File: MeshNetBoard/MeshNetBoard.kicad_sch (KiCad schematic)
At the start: 9 parts, among them J1 Conn_01x02, U1 XIAO-ESP32-S3-DIP, U2 TPS631000DRLR

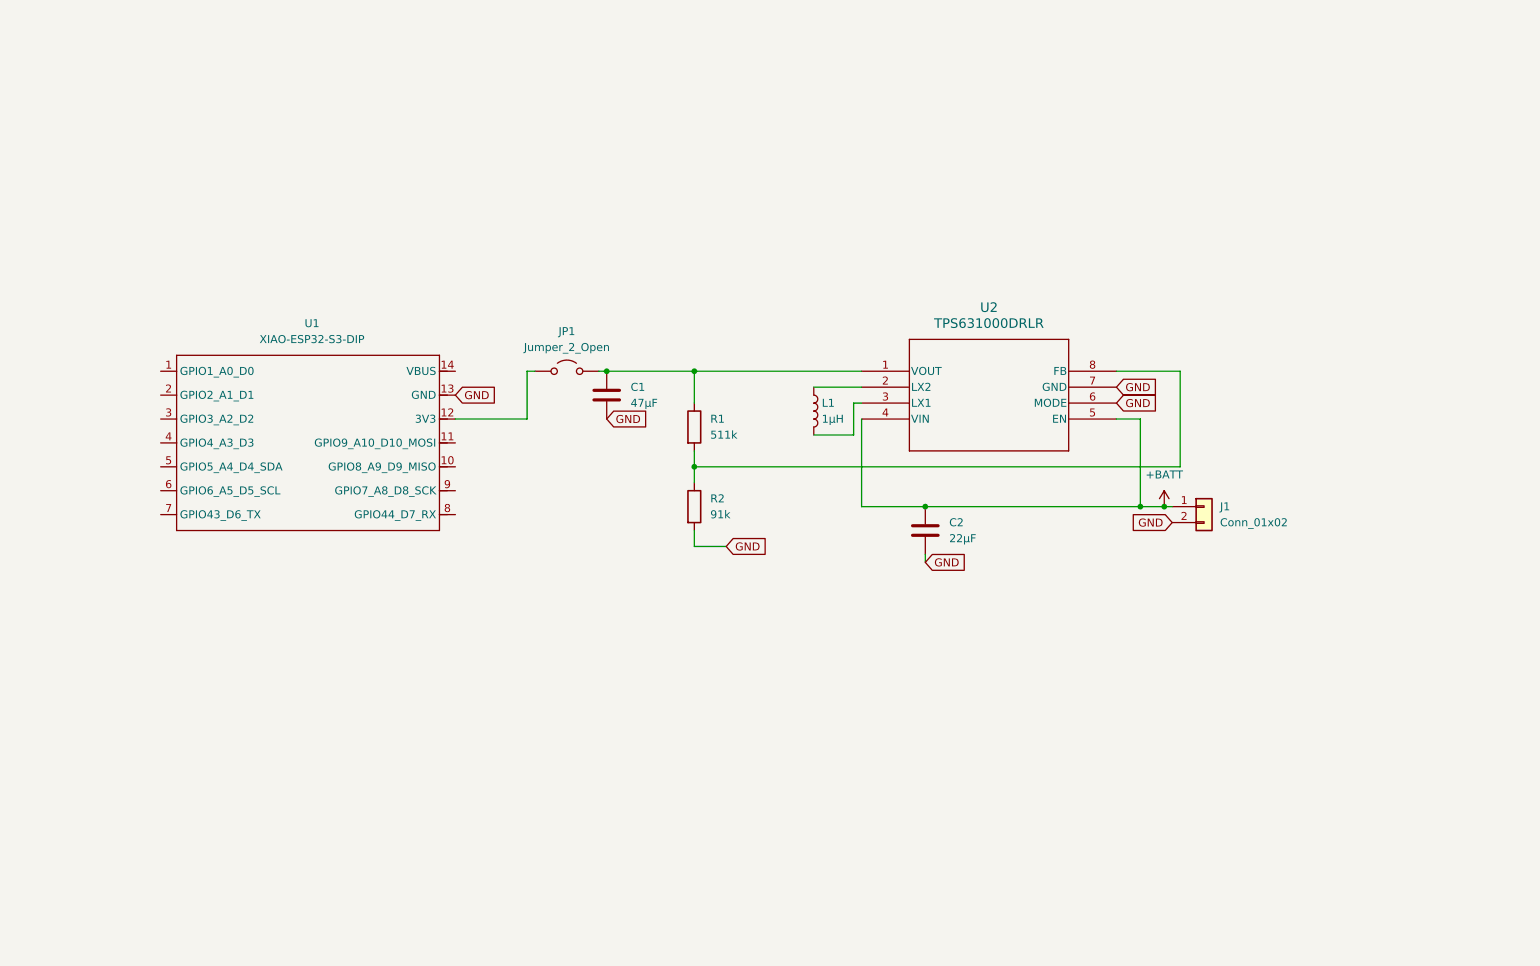
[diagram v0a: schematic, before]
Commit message: for pdr
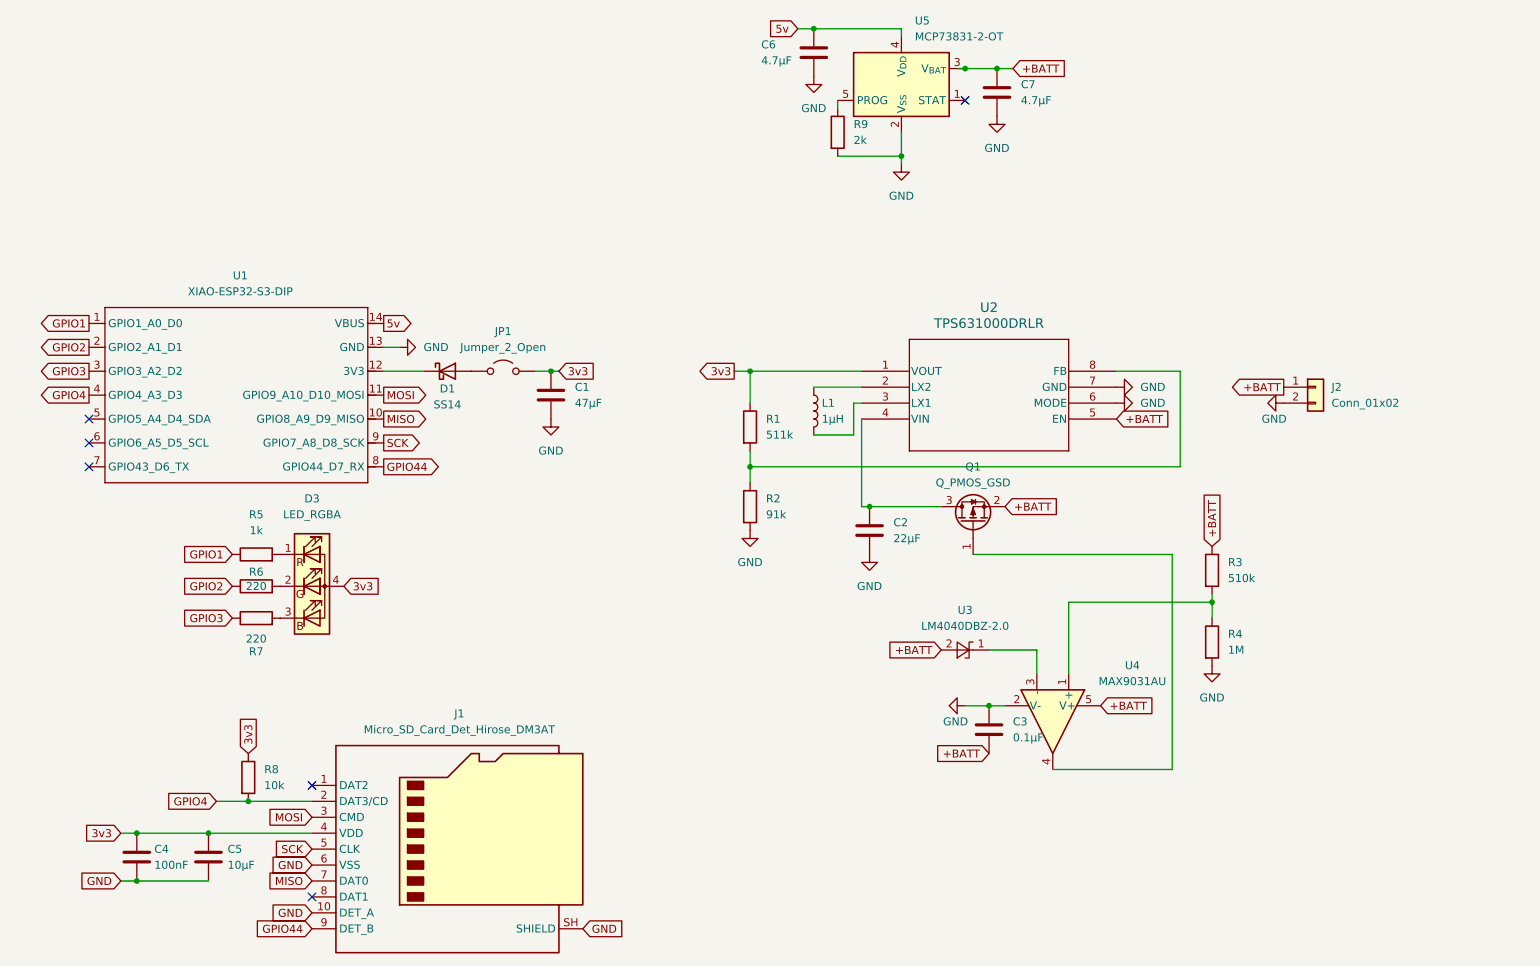
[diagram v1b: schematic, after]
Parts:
- removed J1: Conn_01x02, Connector_JST:JST_PH_S2B-PH-K_1x02_P2.00mm_Horizontal, symbol Connector_Generic:Conn_01x02
- added C3: 0.1μF, Capacitor_SMD:C_0805_2012Metric_Pad1.18x1.45mm_HandSolder, symbol Device:C
- added C4: 100nF, Capacitor_SMD:C_0805_2012Metric_Pad1.18x1.45mm_HandSolder, symbol Device:C
- added C5: 10µF, Capacitor_SMD:C_0805_2012Metric_Pad1.18x1.45mm_HandSolder, symbol Device:C
- added C6, C7: 4.7µF, Capacitor_SMD:C_0805_2012Metric_Pad1.18x1.45mm_HandSolder, symbol Device:C
- added D1: SS14, Diode_SMD:D_SMA, symbol Diode:SS14
- added D3: LED_RGBA, symbol Device:LED_RGBA
- added J1: Micro_SD_Card_Det_Hirose_DM3AT, symbol Connector:Micro_SD_Card_Det_Hirose_DM3AT
- added J2: Conn_01x02, Connector_JST:JST_PH_S2B-PH-K_1x02_P2.00mm_Horizontal, symbol Connector_Generic:Conn_01x02
- added Q1: Q_PMOS_GSD, Package_TO_SOT_SMD:SOT-23, symbol Transistor_FET:Q_PMOS_GSD
- added R3: 510k, Resistor_SMD:R_0805_2012Metric_Pad1.20x1.40mm_HandSolder, symbol Device:R
- added R4: 1M, Resistor_SMD:R_0805_2012Metric_Pad1.20x1.40mm_HandSolder, symbol Device:R
- added R5: 1k, Resistor_SMD:R_0805_2012Metric_Pad1.20x1.40mm_HandSolder, symbol Device:R
- added R6, R7: 220, Resistor_SMD:R_0805_2012Metric_Pad1.20x1.40mm_HandSolder, symbol Device:R
- added R8: 10k, Resistor_SMD:R_0805_2012Metric_Pad1.20x1.40mm_HandSolder, symbol Device:R
- added R9: 2k, Resistor_SMD:R_0805_2012Metric_Pad1.20x1.40mm_HandSolder, symbol Device:R
- added U3: LM4040DBZ-2.0, Package_TO_SOT_SMD:SOT-23, symbol Reference_Voltage:LM4040DBZ-2.0
- added U4: MAX9031AU, Package_TO_SOT_SMD:SOT-23-5, symbol Comparator:MAX9031AU
- added U5: MCP73831-2-OT, Package_TO_SOT_SMD:SOT-23-5, symbol Battery_Management:MCP73831-2-OT
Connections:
- net +BATT: now also C3.2, C7.1, J2.1 (Pin_1), Q1.2 (S), R3.1, U3.2 (A), U4.5 (V+), U5.3 (V_{BAT}); no longer C2.1, U2.4 (VIN)
- net GND: now also C3.1, C4.2, C5.2, C6.2, C7.2, J1.10 (DET_A), J1.6 (VSS), J1.SH (SHIELD), J2.2 (Pin_2), R4.2, R9.2, U4.2 (V-), U5.2 (V_{SS})
- net 3v3: now reaches C1.1, JP1.2 (B), R1.1, U2.1 (VOUT)
- net 3v3: now also C4.1, C5.1, D3.4 (A), J1.4 (VDD), R8.1
- net at U1.12 (3V3): now also D1.1 (K); no longer JP1.1 (A)
- net GPIO1: now reaches U1.1 (GPIO1_A0_D0)
- net GPIO1: now also R5.1
- net MISO: now reaches U1.10 (GPIO8_A9_D9_MISO)
- net MISO: now also J1.7 (DAT0)
- net MOSI: now reaches U1.11 (GPIO9_A10_D10_MOSI)
- net MOSI: now also J1.3 (CMD)
- net 5v: now reaches U1.14 (VBUS)
- net 5v: now also C6.1, U5.4 (V_{DD})
- net GPIO2: now reaches U1.2 (GPIO2_A1_D1)
- net GPIO2: now also R6.1
- net GPIO3: now reaches U1.3 (GPIO3_A2_D2)
- net GPIO3: now also R7.1
- net GPIO4: now reaches U1.4 (GPIO4_A3_D3)
- net GPIO4: now also J1.2 (DAT3/CD), R8.2
- net GPIO44: now reaches U1.8 (GPIO44_D7_RX)
- net GPIO44: now also J1.9 (DET_B)
- net SCK: now reaches U1.9 (GPIO7_A8_D8_SCK)
- net SCK: now also J1.5 (CLK)
- new net: D1.2 (A), JP1.1 (A)
- new net: R3.2, R4.1, U4.1 (+)
- new net: U3.1 (K), U4.3 (-)
- new net: Q1.1 (G), U4.4
- new net: D3.3 (BK), R7.2
- new net: D3.2 (GK), R6.2
- new net: C2.1, Q1.3 (D), U2.4 (VIN)
- new net: R9.1, U5.5 (PROG)
- new net: D3.1 (RK), R5.2
- no-connect marks 0 -> 6
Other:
- moved on the sheet: C1, C2, JP1, R1, R2, U1

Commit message: help me
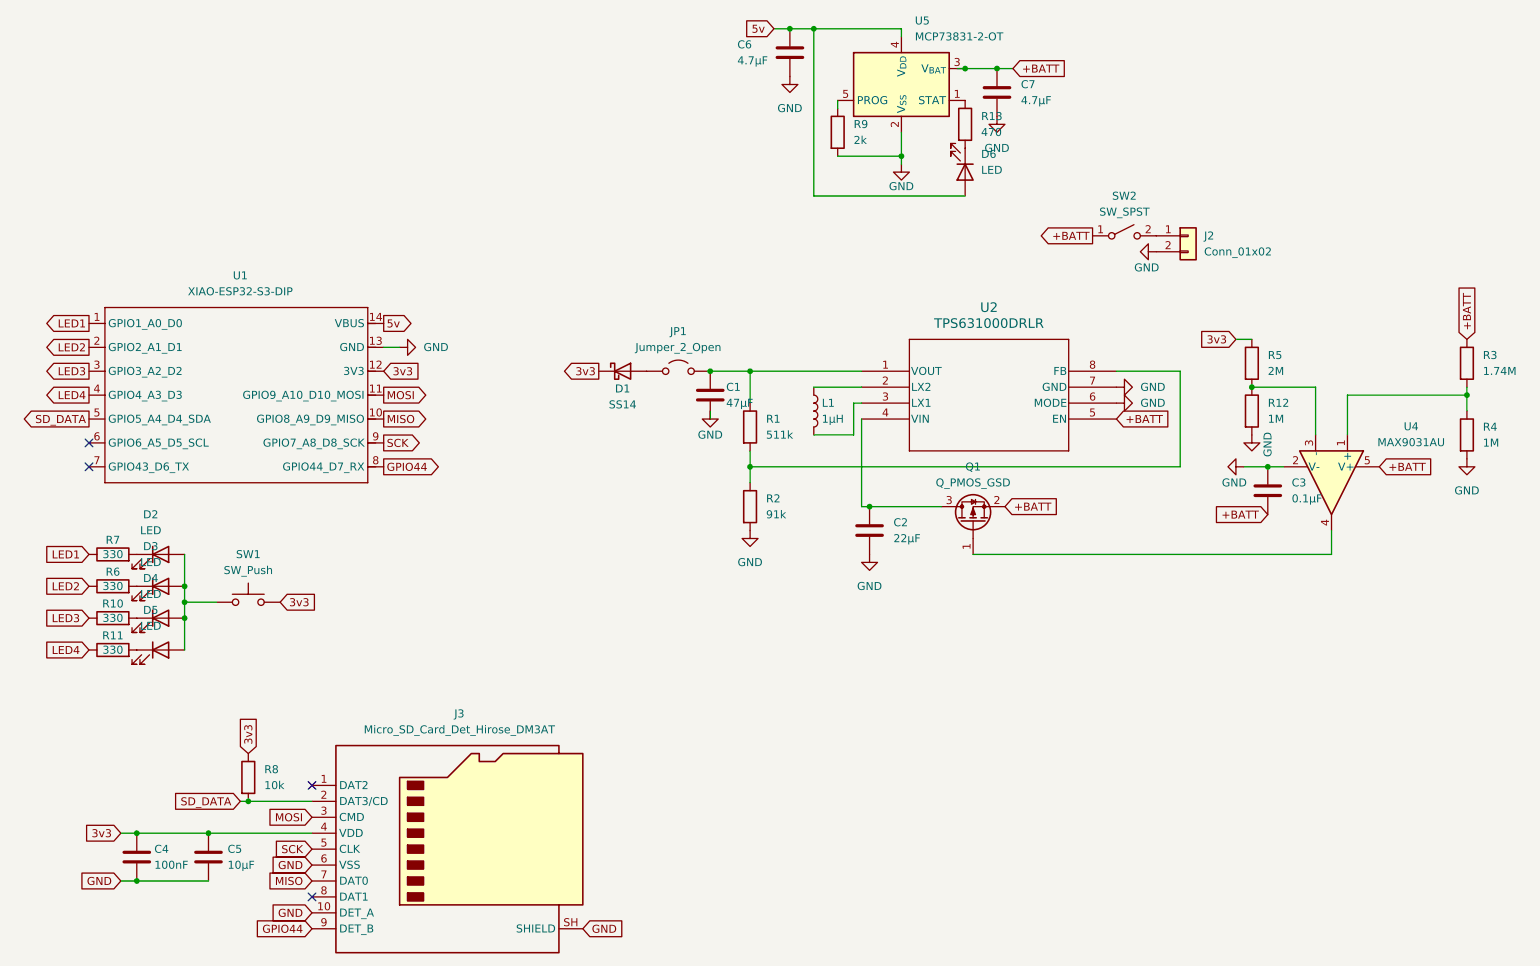
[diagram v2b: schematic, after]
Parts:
- removed D3: LED_RGBA, symbol Device:LED_RGBA
- removed J1: Micro_SD_Card_Det_Hirose_DM3AT, symbol Connector:Micro_SD_Card_Det_Hirose_DM3AT
- removed U3: LM4040DBZ-2.0, Package_TO_SOT_SMD:SOT-23, symbol Reference_Voltage:LM4040DBZ-2.0
- added D2, D3, D4, D5, D6: LED, LED_SMD:LED_1206_3216Metric_Pad1.42x1.75mm_HandSolder, symbol Device:LED
- added J3: Micro_SD_Card_Det_Hirose_DM3AT, Connector_Card:microSD_HC_Hirose_DM3AT-SF-PEJM5, symbol Connector:Micro_SD_Card_Det_Hirose_DM3AT
- added R10, R11: 330, Resistor_SMD:R_0805_2012Metric_Pad1.20x1.40mm_HandSolder, symbol Device:R
- added R12: 1M, Resistor_SMD:R_0805_2012Metric_Pad1.20x1.40mm_HandSolder, symbol Device:R
- added R13: 470, Resistor_SMD:R_0805_2012Metric_Pad1.20x1.40mm_HandSolder, symbol Device:R
- added SW1: SW_Push, Button_Switch_THT:SW_PUSH_6mm_H5mm, symbol Switch:SW_Push
- added SW2: SW_SPST, Button_Switch_THT:SW_Slide_SPDT_Straight_CK_OS102011MS2Q, symbol Switch:SW_SPST
- R3: value 510k -> 1.74M
- R5: value 1k -> 2M
- R6, R7: value 220 -> 330
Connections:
- net +BATT: now also SW2.1 (A); no longer J2.1 (Pin_1)
- net 3v3: now also D1.1 (K), R5.1, U1.12 (3V3), J3.4 (VDD), SW1.2; no longer C1.1, JP1.2 (B), R1.1, U2.1 (VOUT)
- net 5v: now also D6.2 (A)
- net GND: now also J3.10 (DET_A), J3.6 (VSS), J3.SH (SHIELD), R12.2
- net GPIO44: now also J3.9 (DET_B)
- net MISO: now also J3.7 (DAT0)
- net MOSI: now also J3.3 (CMD)
- net SCK: now also J3.5 (CLK)
- net at U4.3 (-): now also R5.2, R12.1
- net at R7.2: now also D2.1 (K)
- net at R6.2: now also D3.1 (K)
- net at U5.1 (STAT): now also R13.1
- net SD_DATA: now reaches U1.5 (GPIO5_A4_D4_SDA)
- net SD_DATA: now also R8.2, J3.2 (DAT3/CD)
- net GPIO1 renamed LED1
- net LED1: now also R7.1; no longer R5.1
- net GPIO2 renamed LED2
- net GPIO3 renamed LED3
- net LED3: now also R10.1; no longer R7.1
- net GPIO4 renamed LED4
- net LED4: now also R11.1; no longer R8.2
- new net: C1.1, JP1.2 (B), R1.1, U2.1 (VOUT)
- new net: D2.2 (A), D3.2 (A), D4.2 (A), D5.2 (A), SW1.1
- new net: D4.1 (K), R10.2
- new net: D6.1 (K), R13.2
- new net: J2.1 (Pin_1), SW2.2 (B)
- new net: D5.1 (K), R11.2
- no-connect marks 6 -> 4
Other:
- moved on the sheet: C1, C3, C6, D1, J2, JP1, R3, R4, R6, U4
